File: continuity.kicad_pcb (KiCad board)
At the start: 2 copper layers, 85 x 35 mm, 28 parts, among them J1 Conn_01x01_Female, J2 Conn_01x04_Female, J3 Conn_01x01_Female, Q1 BCP52, Q2 BCP55, Q3 BCP55, U1 MCP 6V11T-EOT

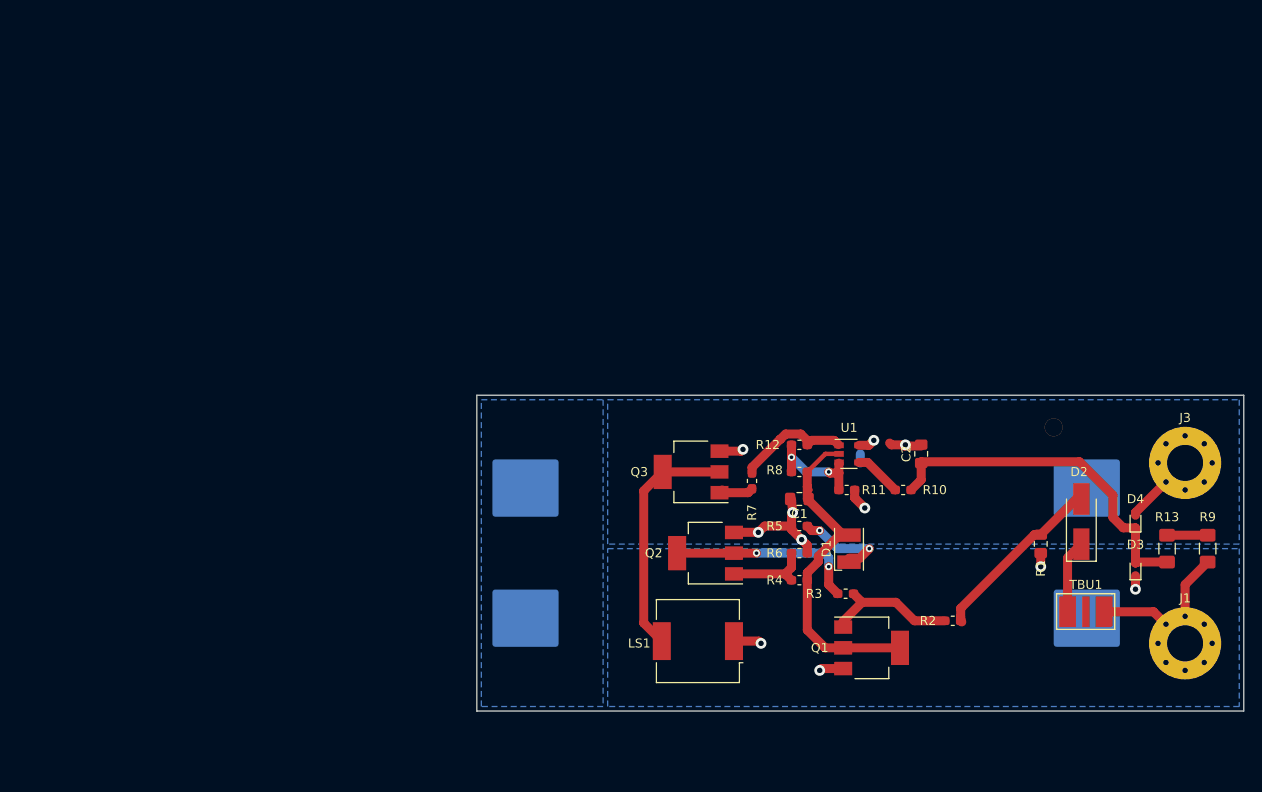
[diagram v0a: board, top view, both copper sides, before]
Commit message: snap
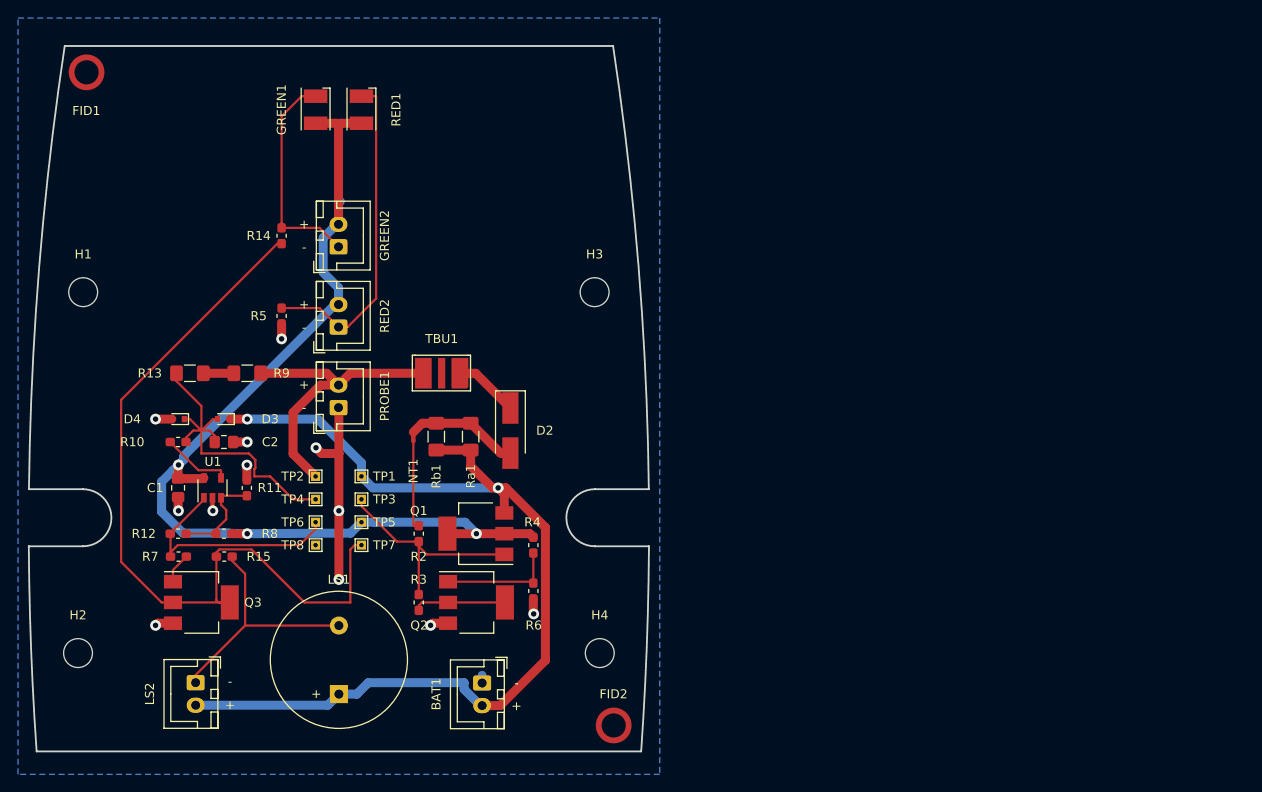
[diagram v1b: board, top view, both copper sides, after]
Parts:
- removed J1, J3: Conn_01x01_Female, MountingHole:MountingHole_4mm_Pad_Via
- removed J2: Conn_01x04_Female, continuity:KEYSTONE_1012
- added BAT1: Conn_01x02_Male, Connector_JST:JST_XH_B2B-XH-A_1x02_P2.50mm_Vertical, F.Cu at (75.6, 96.9)
- added FID1: Fiducial, Fiducial:Fiducial_Modern_CopperTop, F.Cu at (31.8, 29.2)
- added FID2: Fiducial, Fiducial:Fiducial_Modern_CopperTop, F.Cu at (90.2, 101.6)
- added GREEN1: LED, LED_SMD:LED_PLCC-2, F.Cu at (57.1, 33.4)
- added GREEN2: Conn_01x02_Male, Connector_JST:JST_XH_B2B-XH-A_1x02_P2.50mm_Vertical, F.Cu at (59.7, 48.6)
- added H1: MountingHole, MountingHole:MountingHole_3.2mm_M3, F.Cu at (31.4, 53.6)
- added H2: MountingHole, MountingHole:MountingHole_3.2mm_M3, F.Cu at (30.8, 93.6)
- added H3: MountingHole, MountingHole:MountingHole_3.2mm_M3, F.Cu at (88.1, 53.6)
- added H4: MountingHole, MountingHole:MountingHole_3.2mm_M3, F.Cu at (88.6, 93.6)
- added LS2: Conn_01x02_Male, Connector_JST:JST_XH_B2B-XH-A_1x02_P2.50mm_Vertical, F.Cu at (43.8, 96.9)
- added NT1: Net-Tie_2, NetTie:NetTie-2_SMD_Pad0.5mm, F.Cu at (68.0, 69.6)
- added PROBE1: Conn_01x02_Male, Connector_JST:JST_XH_B2B-XH-A_1x02_P2.50mm_Vertical, F.Cu at (59.7, 66.4)
- added R14: 240, Resistor_SMD:R_0603_1608Metric_Pad1.05x0.95mm_HandSolder, F.Cu at (53.4, 47.3)
- added R15: 240, Resistor_SMD:R_0603_1608Metric_Pad1.05x0.95mm_HandSolder, F.Cu at (47.0, 82.9)
- added RED2: Conn_01x02_Male, Connector_JST:JST_XH_B2B-XH-A_1x02_P2.50mm_Vertical, F.Cu at (59.7, 57.4)
- added Ra1: 470, Resistor_SMD:R_1206_3216Metric_Pad1.42x1.75mm_HandSolder, F.Cu at (74.3, 69.6)
- added TP1: VCC, TestPoint:TestPoint_THTPad_1.0x1.0mm_Drill0.5mm, F.Cu at (62.2, 74.0)
- added TP2: PROBE, TestPoint:TestPoint_THTPad_1.0x1.0mm_Drill0.5mm, F.Cu at (57.1, 74.0)
- added TP3: SENSE, TestPoint:TestPoint_THTPad_1.0x1.0mm_Drill0.5mm, F.Cu at (62.2, 76.5)
- added TP4: PROBE_uA, TestPoint:TestPoint_THTPad_1.0x1.0mm_Drill0.5mm, F.Cu at (57.1, 76.5)
- added TP5: VCC_SW, TestPoint:TestPoint_THTPad_1.0x1.0mm_Drill0.5mm, F.Cu at (62.2, 79.1)
- added TP6: KOMP_OUT, TestPoint:TestPoint_THTPad_1.0x1.0mm_Drill0.5mm, F.Cu at (57.1, 79.1)
- added TP7: OUT, TestPoint:TestPoint_THTPad_1.0x1.0mm_Drill0.5mm, F.Cu at (62.2, 81.6)
- added TP8: GND, TestPoint:TestPoint_THTPad_1.0x1.0mm_Drill0.5mm, F.Cu at (57.1, 81.6)
- LS1: footprint Buzzer_Beeper:Buzzer_CUI_CPT-9019S-SMT -> Buzzer_Beeper:Buzzer_15x7.5RM7.6
- R3: value 5k -> 4,7k
- Rb1: renamed from R1; value 240 -> 470; footprint Resistor_SMD:R_0805_2012Metric_Pad1.15x1.40mm_HandSolder -> Resistor_SMD:R_1206_3216Metric_Pad1.42x1.75mm_HandSolder
- moved R13 110.0 mm to (43.2, 62.6), turned to 0 degrees
- moved R9 108.2 mm to (49.6, 62.6), turned to 0 degrees
- moved D4 106.7 mm to (41.9, 67.6), turned to 180 degrees
- moved D3 102.4 mm to (47.0, 67.6), turned to 180 degrees
- moved R10 80.5 mm to (41.9, 70.2)
- moved C2 77.3 mm to (47.0, 70.2), turned to 0 degrees
- moved TBU1 76.1 mm to (71.1, 62.6)
- moved RED1 72.7 mm to (62.2, 33.4), turned to 270 degrees
- moved U1 70.6 mm to (45.7, 75.3), turned to 90 degrees
- moved R12 69.6 mm to (41.9, 80.3), turned to 180 degrees
- moved C1 68.9 mm to (41.9, 75.3), turned to 270 degrees
- moved Rb1 68.0 mm to (70.5, 69.6)
- moved R11 66.5 mm to (49.5, 75.3), turned to 270 degrees
- moved R8 64.1 mm to (47.0, 80.3)
- moved R7 64.1 mm to (41.9, 82.9), turned to 0 degrees
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- renumbered D1 to RED1
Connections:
- net Net-(C2-Pad1) renamed /Probe_uA
- net Net-(J1-Pad1) renamed /Probe
- net Net-(R12-Pad2) renamed /KOMP_OUT
- Q3 pad 2: Net-(LS1-Pad2) -> Net-(Q3-Pad2)
- Q3 pad 4: Net-(LS1-Pad2) -> Net-(Q3-Pad2)
- R2 pad 2: Net-(D2-Pad2) -> Net-(NT1-Pad2)
- U1 pad 2: /VCC_SW -> GND
- U1 pad 5: GND -> /VCC_SW
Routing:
- net /VCC: track 8.79 -> 111.6 mm, vias 4 -> 2
- net Net-(Q3-Pad2): track 0.00 -> 88.4 mm
- net /VCC_SW: track 38.3 -> 114.6 mm, vias 0 -> 3
- net Net-(R5-Pad2): track 10.6 -> 36.7 mm, vias 2 -> 0
- net Net-(GREEN1-Pad1): track 0.00 -> 24.2 mm
- net /KOMP_OUT: track 12.9 -> 26.5 mm
- net /Probe: track 20.5 -> 33.5 mm
- net Net-(Q2-Pad2): track 21.4 -> 10.2 mm, vias 2 -> 0
- net Net-(Q1-Pad1): track 15.0 -> 25.0 mm
- net Net-(NT1-Pad2): track 0.00 -> 9.90 mm
- net Net-(D2-Pad2): track 21.3 -> 12.5 mm
- net GND: track 33.4 -> 38.1 mm, vias 7 -> 12
- net Net-(Q2-Pad1): track 9.25 -> 12.8 mm
- net /Probe_uA: track 39.3 -> 35.7 mm
- net Net-(R10-Pad1): track 5.29 -> 7.74 mm
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- removed copper zone on B.Cu, net /VCC
- removed copper zone on B.Cu, net Net-(J2-Pad2)
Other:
- board size 85 x 35 mm -> 68.7 x 78.2 mm
- net class Probe added: clearance 0.8, trace_width 1, via_dia 1.2, via_drill 0.6
- rule trace_min: 0.2 -> 0
- board text added: "+"
- board text added: "-"

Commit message: snap
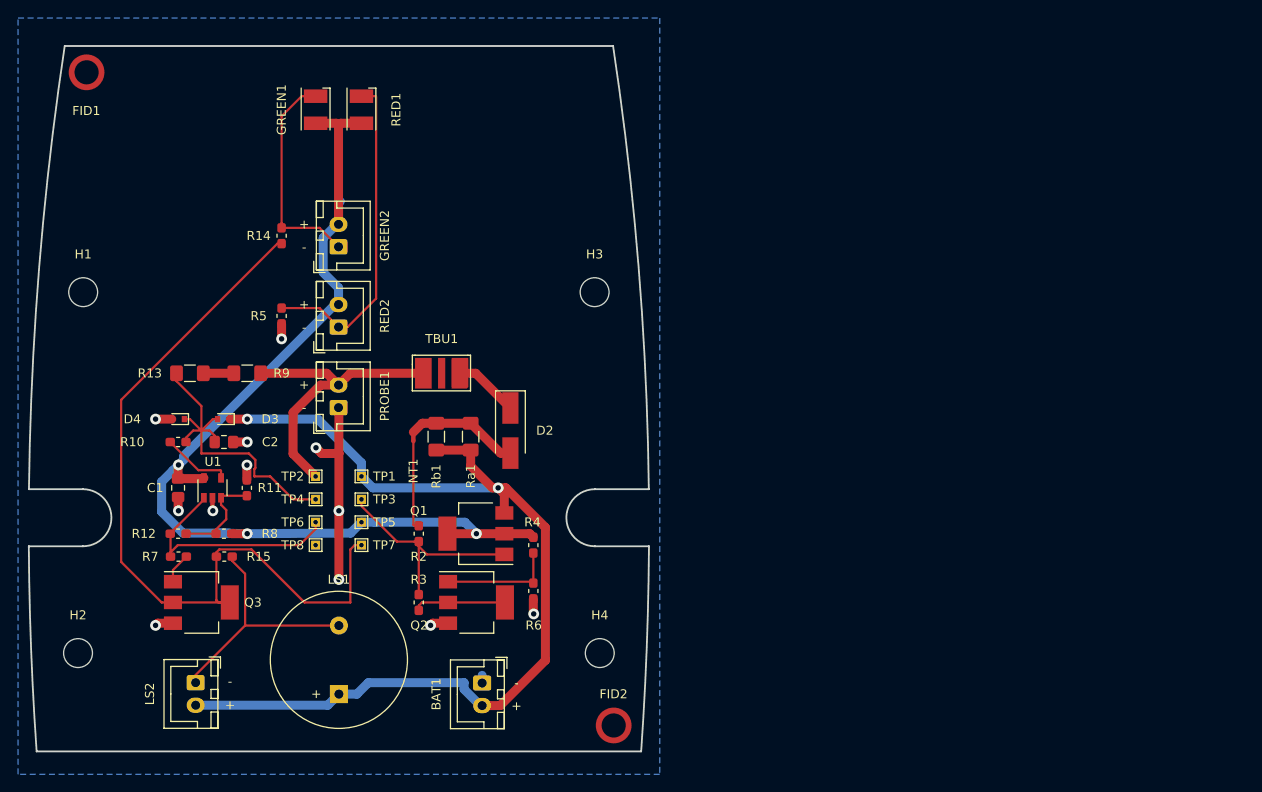
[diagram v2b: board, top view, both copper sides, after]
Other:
- net class Default removed
- net class Power removed
- net class Probe removed
